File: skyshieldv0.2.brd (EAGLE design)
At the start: 17.8 x 43.2 mm, 21 parts, among them IC2 MCP1702-5, J1 HEAD15-NOSS, J2 HEAD15-NOSS-1

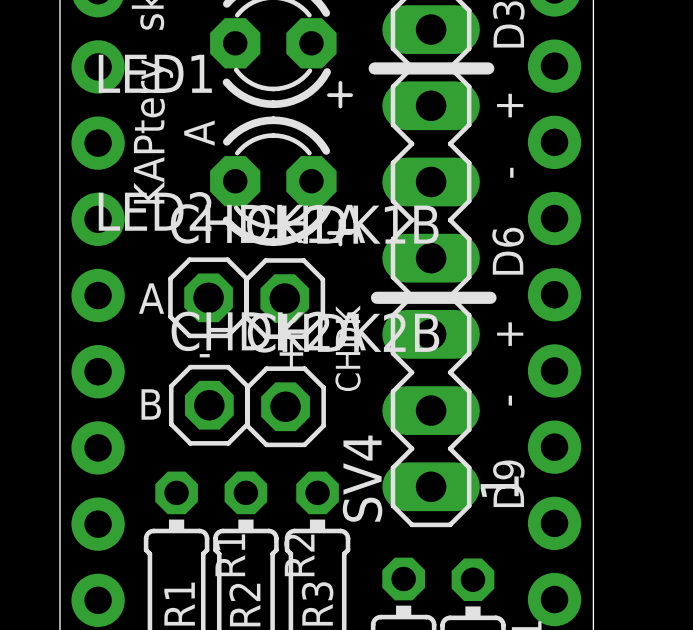
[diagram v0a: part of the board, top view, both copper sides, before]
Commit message: update
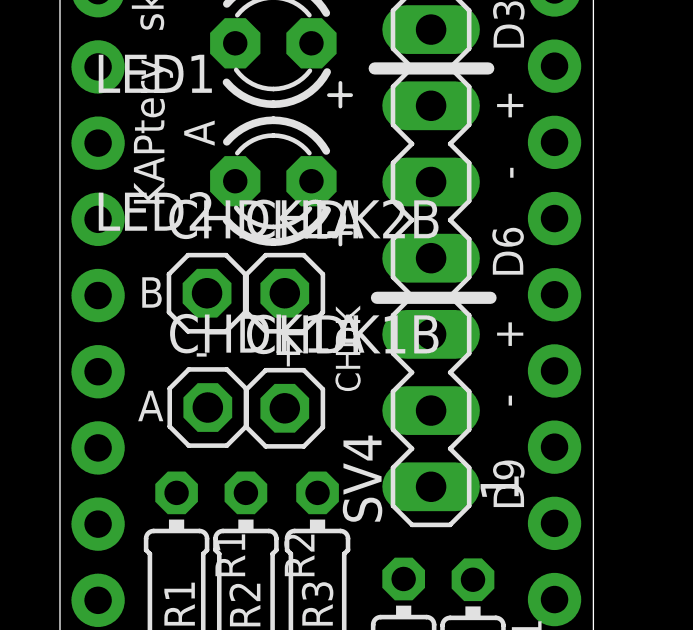
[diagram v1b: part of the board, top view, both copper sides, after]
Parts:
- R1, R2, R3: value 1.5K -> 10K
- moved CHDK2B 3.78 mm to (7.49, 19.1)
- moved CHDK2A 3.73 mm to (4.90, 19.1)
- moved CHDK1A 3.66 mm to (4.93, 15.3)
- moved CHDK1B 3.66 mm to (7.49, 15.3)
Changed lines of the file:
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@@
 <wire x1="10.4902" y1="26.5938" x2="14.2748" y2="26.5938" width="0.4064" layer="21"/>
 <wire x1="10.5664" y1="18.9484" x2="14.351" y2="18.9484" width="0.4064" layer="21"/>
-<text x="4.5974" y="16.637" size="1.016" layer="21" ratio="15">-</text>
+<text x="4.4958" y="16.6624" size="1.016" layer="21" ratio="15">-</text>
 <text x="9.1948" y="18.669" size="0.8128" layer="21" ratio="15" rot="R270">CHDK</text>
-<text x="7.1882" y="16.637" size="1.016" layer="21" ratio="15">+</text>
-<text x="3.4798" y="19.431" size="1.016" layer="21" ratio="15" rot="R180">A</text>
-<text x="3.4544" y="15.9004" size="1.016" layer="21" ratio="15" rot="R180">B</text>
+<text x="7.0866" y="16.6624" size="1.016" layer="21" ratio="15">+</text>
+<text x="3.4544" y="15.8496" size="1.016" layer="21" ratio="15" rot="R180">A</text>
+<text x="3.4798" y="19.6342" size="1.016" layer="21" ratio="15" rot="R180">B</text>
 <text x="2.4892" y="1.5494" size="1.016" layer="21" ratio="15">S</text>
 <text x="4.4958" y="7.8994" size="1.016" layer="21" ratio="15" rot="R90">R1</text>
@@
 <element name="J1" library="MyCON2" package="HEAD15-NOSS" value="HEAD15-NOSS" x="16.4846" y="39.37" rot="R270"/>
 <element name="J2" library="MyCON2" package="HEAD15-NOSS-1" value="HEAD15-NOSS-1" x="1.27" y="39.3446" rot="R270"/>
-<element name="R1" library="rcl" package="0204/7" value="1.5K" x="3.8862" y="8.636" rot="R270"/>
+<element name="R1" library="rcl" package="0204/7" value="10K" x="3.8862" y="8.636" rot="R270"/>
 <element name="IC2" library="JeeLabs" package="TO92" value="MCP1702-5" x="6.6294" y="36.0426"/>
 <element name="C5" library="resistor" package="E1,8-4" value="10µ" x="12.4206" y="36.9824" rot="R90"/>
@@
 <attribute name="VALUE" x="15.2908" y="22.8092" size="1.27" layer="27" ratio="10" rot="R90"/>
 </element>
-<element name="R2" library="rcl" package="0204/7" value="1.5K" x="6.1976" y="8.636" rot="R270"/>
+<element name="R2" library="rcl" package="0204/7" value="10K" x="6.1976" y="8.636" rot="R270"/>
 <element name="LED1" library="adafruit" package="LED3MM" value="POWERLED" x="7.112" y="27.432" rot="R180"/>
-<element name="R3" library="rcl" package="0204/7" value="1.5K" x="8.5852" y="8.636" rot="R90"/>
+<element name="R3" library="rcl" package="0204/7" value="10K" x="8.5852" y="8.636" rot="R90"/>
 <element name="LED2" library="adafruit" package="LED3MM" value="POWERLED" x="7.112" y="22.8346" rot="R180"/>
 <element name="RS2" library="rcl" package="0204/7" value="10K" x="11.4554" y="5.7658" rot="R90"/>
 <element name="RS1" library="rcl" package="0204/7" value="100" x="13.7668" y="5.7404" rot="R270"/>
-<element name="CHDK1A" library="pinhead" package="1X01" value="" x="4.953" y="18.9484"/>
-<element name="CHDK1B" library="pinhead" package="1X01" value="" x="7.493" y="18.923"/>
-<element name="CHDK2A" library="pinhead" package="1X01" value="" x="4.9784" y="15.367"/>
-<element name="CHDK2B" library="pinhead" package="1X01" value="" x="7.5184" y="15.3162"/>
+<element name="CHDK1A" library="pinhead" package="1X01" value="" x="4.9276" y="15.2908"/>
+<element name="CHDK1B" library="pinhead" package="1X01" value="" x="7.493" y="15.2654"/>
+<element name="CHDK2A" library="pinhead" package="1X01" value="" x="4.9022" y="19.1008"/>
+<element name="CHDK2B" library="pinhead" package="1X01" value="" x="7.493" y="19.1008"/>
 <element name="SW1B" library="pinhead" package="1X01" value="" x="5.0038" y="2.1336"/>
 <element name="SW1A" library="pinhead" package="1X01" value="" x="7.5692" y="2.159"/>
@@
 <wire x1="5.842" y1="27.432" x2="5.8674" y2="31.9278" width="0" layer="19" extent="1-1"/>
 <wire x1="5.842" y1="22.8346" x2="5.842" y2="27.432" width="0" layer="19" extent="1-1"/>
-<wire x1="7.493" y1="18.923" x2="5.842" y2="22.8346" width="0" layer="19" extent="1-1"/>
-<wire x1="7.5184" y1="15.3162" x2="7.493" y2="18.923" width="0" layer="19" extent="1-1"/>
+<wire x1="7.493" y1="15.2654" x2="5.842" y2="22.8346" width="0" layer="19" extent="1-1"/>
+<wire x1="7.493" y1="19.1008" x2="7.493" y2="15.2654" width="0" layer="19" extent="1-1"/>
 <wire x1="5.5372" y1="40.8686" x2="5.3594" y2="36.0426" width="0" layer="19" extent="1-1"/>
-<wire x1="12.3698" y1="17.7292" x2="7.493" y2="18.923" width="0" layer="19" extent="1-1"/>
+<wire x1="12.3698" y1="17.7292" x2="7.493" y2="15.2654" width="0" layer="19" extent="1-1"/>
 <wire x1="12.3698" y1="25.3492" x2="5.842" y2="27.432" width="0" layer="19" extent="1-1"/>
-<wire x1="5.0038" y1="2.1336" x2="7.5184" y2="15.3162" width="0" layer="19" extent="1-1"/>
+<wire x1="5.0038" y1="2.1336" x2="7.493" y2="19.1008" width="0" layer="19" extent="1-1"/>
 </signal>
 <signal name="VCC" class="1">
@@
 <contactref element="J2" pad="11"/>
 <contactref element="CHDK2A" pad="1"/>
-<wire x1="1.27" y1="13.9446" x2="4.9784" y2="15.367" width="0" layer="19" extent="1-1"/>
+<wire x1="1.27" y1="13.9446" x2="4.9022" y2="19.1008" width="0" layer="19" extent="1-1"/>
 </signal>
 <signal name="A0">
 <contactref element="J2" pad="12"/>
 <contactref element="CHDK1A" pad="1"/>
-<wire x1="1.27" y1="11.4046" x2="4.953" y2="18.9484" width="0" layer="19" extent="1-1"/>
+<wire x1="1.27" y1="11.4046" x2="4.9276" y2="15.2908" width="0" layer="19" extent="1-1"/>
 </signal>
 <signal name="N$5">
